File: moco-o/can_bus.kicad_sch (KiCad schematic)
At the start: 10 parts, among them J11 Conn_02x02_Top_Bottom, J12 Conn_02x02_Top_Bottom, U5 TJA1051T-3

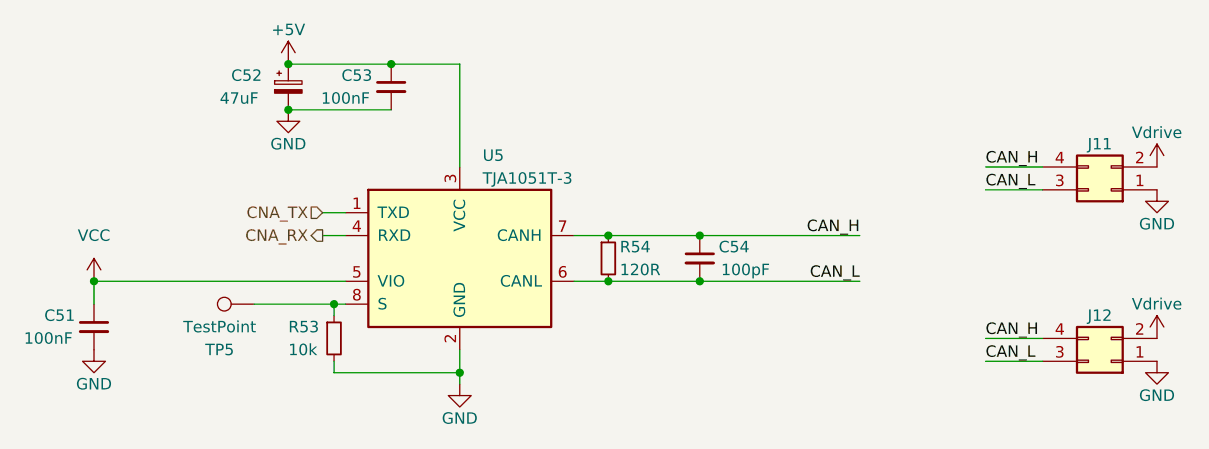
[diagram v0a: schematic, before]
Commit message: Move files
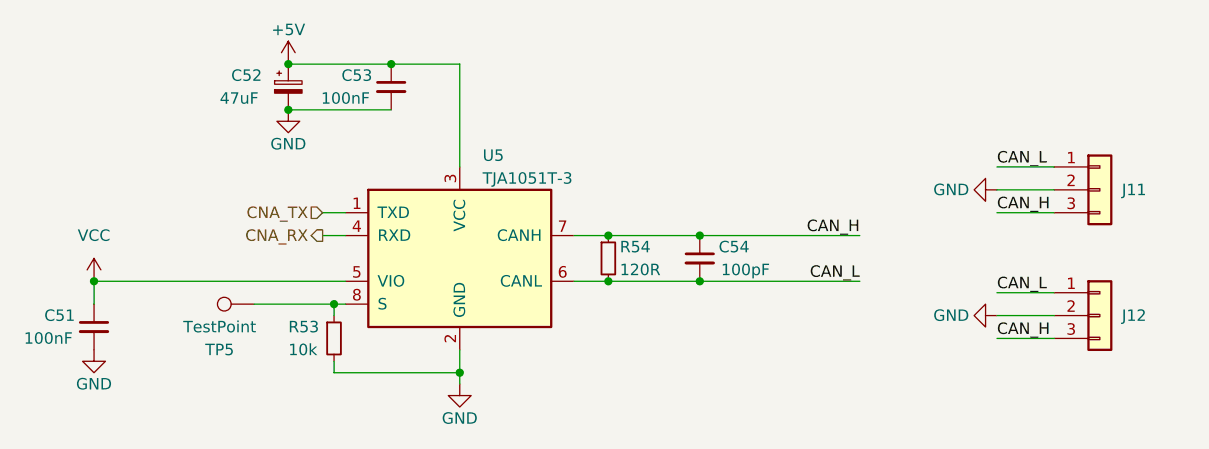
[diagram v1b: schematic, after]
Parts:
- removed J12: Conn_02x02_Top_Bottom, moco:Molex 43045-0406 Micro-Fit 3.0 2x02P, symbol Connector_Generic:Conn_02x02_Top_Bottom
- added J12: Conn_02x02_Top_Bottom, Connector_JST:JST_GH_SM03B-GHS-TB_1x03-1MP_P1.25mm_Horizontal, symbol Connector_Generic:Conn_01x03
- J11: footprint moco:Molex 43045-0406 Micro-Fit 3.0 2x02P -> Connector_JST:JST_GH_SM03B-GHS-TB_1x03-1MP_P1.25mm_Horizontal; symbol Connector_Generic:Conn_02x02_Top_Bottom -> Connector_Generic:Conn_01x03; JLCPCB Part # C505218 -> (none); MFR.Part # 430450406 -> (none)
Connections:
- net Vdrive is gone; now on net GND: J11.2 (Pin_2)
- net CAN_H: now also J11.3 (Pin_3), J12.3 (Pin_3); no longer J11.4 (Pin_4)
- net CAN_L: now also J11.1 (Pin_1), J12.1 (Pin_1); no longer J11.3 (Pin_3)
- net GND: now also J12.2 (Pin_2); no longer J11.1 (Pin_1)
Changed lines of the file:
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@@
   (junction (at 110.49 118.11) (diameter 0) (color 0 0 0 0)
   )
-  (wire (pts (xy 182.88 124.46) (xy 189.23 124.46))
-    (stroke (width 0) (type default) (color 0 0 0 0))
-  )
   (wire (pts (xy 124.46 91.44) (xy 124.46 102.87))
     (stroke (width 0) (type default) (color 0 0 0 0))
@@
     (stroke (width 0) (type default) (color 0 0 0 0))
   )
-  (wire (pts (xy 182.88 102.87) (xy 189.23 102.87))
-    (stroke (width 0) (type default) (color 0 0 0 0))
-  )
   (wire (pts (xy 124.46 125.73) (xy 110.49 125.73))
     (stroke (width 0) (type default) (color 0 0 0 0))
   )
-  (wire (pts (xy 182.88 121.92) (xy 189.23 121.92))
-    (stroke (width 0) (type default) (color 0 0 0 0))
-  )
   (wire (pts (xy 110.49 125.73) (xy 110.49 124.46))
     (stroke (width 0) (type default) (color 0 0 0 0))
@@
     (stroke (width 0) (type default) (color 0 0 0 0))
   )
+  (wire (pts (xy 184.15 119.38) (xy 190.5 119.38))
+    (stroke (width 0) (type default) (color 0 0 0 0))
+  )
+  (wire (pts (xy 184.15 102.87) (xy 190.5 102.87))
+    (stroke (width 0) (type default) (color 0 0 0 0))
+  )
   (wire (pts (xy 105.41 96.52) (xy 116.84 96.52))
     (stroke (width 0) (type default) (color 0 0 0 0))
@@
     (stroke (width 0) (type default) (color 0 0 0 0))
   )
+  (wire (pts (xy 184.15 105.41) (xy 190.5 105.41))
+    (stroke (width 0) (type default) (color 0 0 0 0))
+  )
   (wire (pts (xy 116.84 91.44) (xy 124.46 91.44))
     (stroke (width 0) (type default) (color 0 0 0 0))
@@
     (stroke (width 0) (type default) (color 0 0 0 0))
   )
-  (wire (pts (xy 182.88 105.41) (xy 189.23 105.41))
+  (wire (pts (xy 184.15 116.84) (xy 190.5 116.84))
     (stroke (width 0) (type default) (color 0 0 0 0))
   )
@@
     (stroke (width 0) (type default) (color 0 0 0 0))
   )
+  (wire (pts (xy 184.15 107.95) (xy 190.5 107.95))
+    (stroke (width 0) (type default) (color 0 0 0 0))
+  )
   (wire (pts (xy 137.16 110.49) (xy 140.97 110.49))
     (stroke (width 0) (type default) (color 0 0 0 0))
@@
     (stroke (width 0) (type default) (color 0 0 0 0))
   )
+  (wire (pts (xy 184.15 121.92) (xy 190.5 121.92))
+    (stroke (width 0) (type default) (color 0 0 0 0))
+  )
   (wire (pts (xy 83.82 118.11) (xy 83.82 115.57))
     (stroke (width 0) (type default) (color 0 0 0 0))
@@
     (stroke (width 0) (type default) (color 0 0 0 0))
   )
-  (label "CAN_L" (at 182.88 124.46 0)
+  (label "CAN_H" (at 184.15 121.92 0)
     (effects (font (size 1.27 1.27)) (justify left bottom))
   )
@@
     (effects (font (size 1.27 1.27)) (justify right bottom))
   )
-  (label "CAN_H" (at 182.88 121.92 0)
+  (label "CAN_L" (at 184.15 102.87 0)
     (effects (font (size 1.27 1.27)) (justify left bottom))
   )
@@
     (effects (font (size 1.27 1.27)) (justify right bottom))
   )
-  (label "CAN_H" (at 182.88 102.87 0)
+  (label "CAN_H" (at 184.15 107.95 0)
     (effects (font (size 1.27 1.27)) (justify left bottom))
   )
-  (label "CAN_L" (at 182.88 105.41 0)
+  (label "CAN_L" (at 184.15 116.84 0)
     (effects (font (size 1.27 1.27)) (justify left bottom))
   )
@@
     (pin "8")
   )
+  (symbol (lib_id "power:GND") (at 184.15 119.38 270) (unit 1)
+    (in_bom yes) (on_board yes)
+    (property "Reference" "#PWR0103" (id 0) (at 177.8 119.38 0)
+      (effects (font (size 1.27 1.27)) hide)
+    )
+    (property "Value" "GND" (id 1) (at 179.07 119.38 90))
+    (property "Footprint" "" (id 2) (at 184.15 119.38 0)
+      (effects (font (size 1.27 1.27)) hide)
+    )
+    (property "Datasheet" "" (id 3) (at 184.15 119.38 0)
+      (effects (font (size 1.27 1.27)) hide)
+    )
+    (pin "1")
+  )
   (symbol (lib_id "Connector:TestPoint") (at 101.6 118.11 90) (unit 1)
     (in_bom no) (on_board yes)
@@
     (pin "1")
   )
+  (symbol (lib_id "power:GND") (at 184.15 105.41 270) (unit 1)
+    (in_bom yes) (on_board yes)
+    (property "Reference" "#PWR0102" (id 0) (at 177.8 105.41 0)
+      (effects (font (size 1.27 1.27)) hide)
+    )
+    (property "Value" "GND" (id 1) (at 179.07 105.41 90))
+    (property "Footprint" "" (id 2) (at 184.15 105.41 0)
+      (effects (font (size 1.27 1.27)) hide)
+    )
+    (property "Datasheet" "" (id 3) (at 184.15 105.41 0)
+      (effects (font (size 1.27 1.27)) hide)
+    )
+    (pin "1")
+  )
   (symbol (lib_id "power:+5V") (at 105.41 91.44 0) (unit 1)
     (in_bom yes) (on_board yes)
@@
     (pin "2")
   )
-  (symbol (lib_id "power:GND") (at 201.93 124.46 0) (unit 1)
-    (in_bom yes) (on_board yes)
-    (property "Reference" "#PWR0105" (id 0) (at 201.93 130.81 0)
-      (effects (font (size 1.27 1.27)) hide)
-    )
-    (property "Value" "GND" (id 1) (at 201.93 128.27 0))
-    (property "Footprint" "" (id 2) (at 201.93 124.46 0)
-      (effects (font (size 1.27 1.27)) hide)
-    )
-    (property "Datasheet" "" (id 3) (at 201.93 124.46 0)
-      (effects (font (size 1.27 1.27)) hide)
-    )
-    (pin "1")
-  )
-  (symbol (lib_id "power:Vdrive") (at 201.93 121.92 0) (unit 1)
-    (in_bom yes) (on_board yes)
-    (property "Reference" "#PWR0104" (id 0) (at 196.85 125.73 0)
-      (effects (font (size 1.27 1.27)) hide)
-    )
-    (property "Value" "Vdrive" (id 1) (at 201.93 118.11 0))
-    (property "Footprint" "" (id 2) (at 201.93 121.92 0)
-      (effects (font (size 1.27 1.27)) hide)
-    )
-    (property "Datasheet" "" (id 3) (at 201.93 121.92 0)
-      (effects (font (size 1.27 1.27)) hide)
-    )
-    (pin "1")
-  )
-  (symbol (lib_id "Connector_Generic:Conn_02x02_Top_Bottom") (at 196.85 105.41 180) (unit 1)
-    (in_bom yes) (on_board yes)
-    (property "Reference" "J11" (id 0) (at 195.58 100.33 0))
-    (property "Value" "Conn_02x02_Top_Bottom" (id 1) (at 195.58 99.06 0)
-      (effects (font (size 1.27 1.27)) hide)
-    )
-    (property "Footprint" "moco:Molex 43045-0406 Micro-Fit 3.0 2x02P" (id 2) (at 196.85 105.41 0)
-      (effects (font (size 1.27 1.27)) hide)
-    )
-    (property "Datasheet" "~" (id 3) (at 196.85 105.41 0)
-      (effects (font (size 1.27 1.27)) hide)
-    )
-    (property "JLCPCB Part #" "C505218" (id 4) (at 196.85 105.41 0)
-      (effects (font (size 1.27 1.27)) hide)
-    )
-    (property "MFR.Part #" "430450406" (id 5) (at 196.85 105.41 0)
+  (symbol (lib_id "Connector_Generic:Conn_01x03") (at 195.58 105.41 0) (unit 1)
+    (in_bom yes) (on_board yes)
+    (property "Reference" "J11" (id 0) (at 199.39 105.41 0))
+    (property "Value" "Conn_02x02_Top_Bottom" (id 1) (at 196.85 111.76 0)
+      (effects (font (size 1.27 1.27)) hide)
+    )
+    (property "Footprint" "Connector_JST:JST_GH_SM03B-GHS-TB_1x03-1MP_P1.25mm_Horizontal" (id 2) (at 195.58 105.41 0)
+      (effects (font (size 1.27 1.27)) hide)
+    )
+    (property "Datasheet" "~" (id 3) (at 195.58 105.41 0)
+      (effects (font (size 1.27 1.27)) hide)
+    )
+    (property "JLCPCB Part #" "" (id 4) (at 195.58 105.41 0)
+      (effects (font (size 1.27 1.27)) hide)
+    )
+    (property "MFR.Part #" "" (id 5) (at 195.58 105.41 0)
       (effects (font (size 1.27 1.27)) hide)
     )
@@
     (pin "2")
     (pin "3")
-    (pin "4")
-  )
-  (symbol (lib_id "power:GND") (at 201.93 105.41 0) (unit 1)
-    (in_bom yes) (on_board yes)
-    (property "Reference" "#PWR0103" (id 0) (at 201.93 111.76 0)
-      (effects (font (size 1.27 1.27)) hide)
-    )
-    (property "Value" "GND" (id 1) (at 201.93 109.22 0))
-    (property "Footprint" "" (id 2) (at 201.93 105.41 0)
-      (effects (font (size 1.27 1.27)) hide)
-    )
-    (property "Datasheet" "" (id 3) (at 201.93 105.41 0)
-      (effects (font (size 1.27 1.27)) hide)
-    )
-    (pin "1")
+  )
+  (symbol (lib_id "Connector_Generic:Conn_01x03") (at 195.58 119.38 0) (unit 1)
+    (in_bom yes) (on_board yes)
+    (property "Reference" "J12" (id 0) (at 199.39 119.38 0))
+    (property "Value" "Conn_02x02_Top_Bottom" (id 1) (at 196.85 125.73 0)
+      (effects (font (size 1.27 1.27)) hide)
+    )
+    (property "Footprint" "Connector_JST:JST_GH_SM03B-GHS-TB_1x03-1MP_P1.25mm_Horizontal" (id 2) (at 195.58 119.38 0)
+      (effects (font (size 1.27 1.27)) hide)
+    )
+    (property "Datasheet" "~" (id 3) (at 195.58 119.38 0)
+      (effects (font (size 1.27 1.27)) hide)
+    )
+    (property "JLCPCB Part #" "" (id 4) (at 195.58 119.38 0)
+      (effects (font (size 1.27 1.27)) hide)
+    )
+    (property "MFR.Part #" "" (id 5) (at 195.58 119.38 0)
+      (effects (font (size 1.27 1.27)) hide)
+    )
+    (pin "1")
+    (pin "2")
+    (pin "3")
   )
   (symbol (lib_id "Device:C_Small") (at 83.82 120.65 0) (unit 1)
@@
     (pin "2")
   )
-  (symbol (lib_id "Connector_Generic:Conn_02x02_Top_Bottom") (at 196.85 124.46 180) (unit 1)
-    (in_bom yes) (on_board yes)
-    (property "Reference" "J12" (id 0) (at 195.58 119.38 0))
-    (property "Value" "Conn_02x02_Top_Bottom" (id 1) (at 195.58 118.11 0)
-      (effects (font (size 1.27 1.27)) hide)
-    )
-    (property "Footprint" "moco:Molex 43045-0406 Micro-Fit 3.0 2x02P" (id 2) (at 196.85 124.46 0)
-      (effects (font (size 1.27 1.27)) hide)
-    )
-    (property "Datasheet" "~" (id 3) (at 196.85 124.46 0)
-      (effects (font (size 1.27 1.27)) hide)
-    )
-    (property "JLCPCB Part #" "C505218" (id 4) (at 196.85 124.46 0)
-      (effects (font (size 1.27 1.27)) hide)
-    )
-    (property "MFR.Part #" "430450406" (id 5) (at 196.85 124.46 0)
-      (effects (font (size 1.27 1.27)) hide)
-    )
-    (pin "1")
-    (pin "2")
-    (pin "3")
-    (pin "4")
-  )
-  (symbol (lib_id "power:Vdrive") (at 201.93 102.87 0) (unit 1)
-    (in_bom yes) (on_board yes)
-    (property "Reference" "#PWR0102" (id 0) (at 196.85 106.68 0)
-      (effects (font (size 1.27 1.27)) hide)
-    )
-    (property "Value" "Vdrive" (id 1) (at 201.93 99.06 0))
-    (property "Footprint" "" (id 2) (at 201.93 102.87 0)
-      (effects (font (size 1.27 1.27)) hide)
-    )
-    (property "Datasheet" "" (id 3) (at 201.93 102.87 0)
-      (effects (font (size 1.27 1.27)) hide)
-    )
-    (pin "1")
-  )
 )
